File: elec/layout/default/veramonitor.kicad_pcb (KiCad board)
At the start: 2 copper layers, 111.2 x 70.4 mm, 109 parts, among them J1 ?, U1 ?, U10 ?, U11 ?, U12 ?, U13 ?, U14 ?, U15 ?, U16 ?, U17 ?, U18 ?, U19 ?, U2 ?, U20 ?, U21 ?, U22 ?, U23 ?, U24 ?, U25 ?, U26 ?, U27 ?, U28 ?, U29 ?, U3 ?, U30 ?, U31 ?, U32 ?, U33 ?, U34 ?, U35 ?, U36 ?, U37 ?, U38 ?, U39 ?, U4 ?, U40 ?, U41 ?, U42 ?, U43 ?, U44 ?, U45 ?, U46 ?, U47 ?, U48 ?, U49 ?, U5 ?, U50 ?, U51 ?, U6 ?, U7 ?, U8 ?, U9 ?

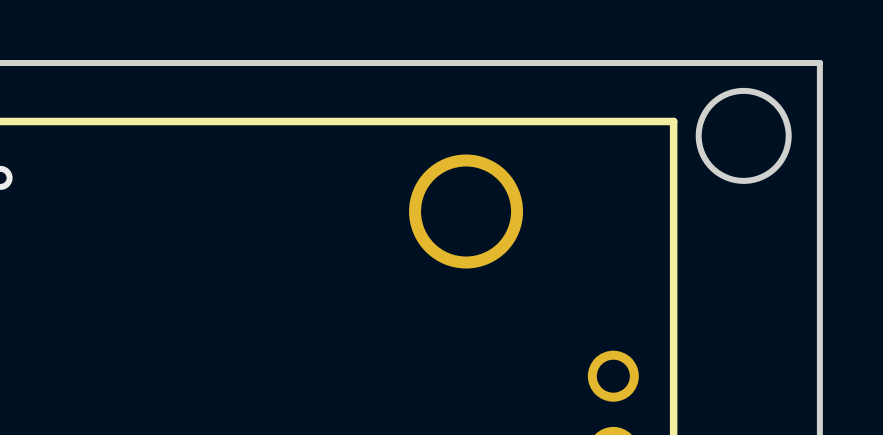
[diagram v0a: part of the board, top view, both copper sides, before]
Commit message: probs done
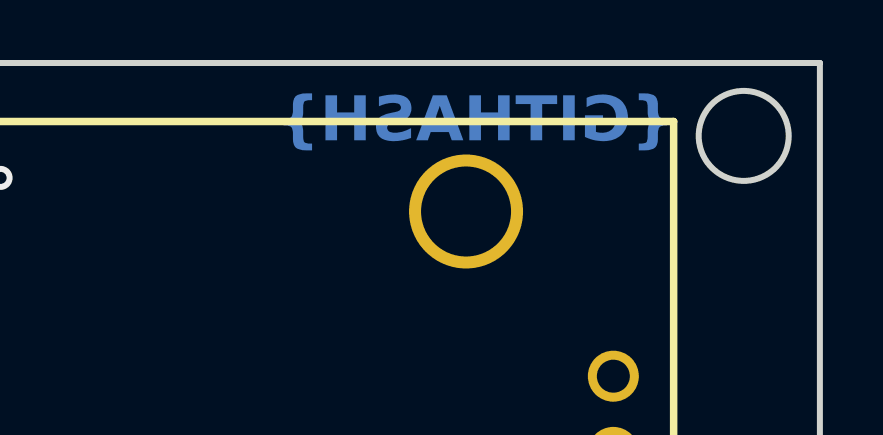
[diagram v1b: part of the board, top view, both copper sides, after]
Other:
- board text added: "{GITHASH}"
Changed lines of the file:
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@@
 		(layer "Edge.Cuts")
+	)
+	(gr_text "{GITHASH}"
+		(at 146.47 69.66 -0)
+		(layer "B.Cu")
+		(effects
+			(font
+				(size 1.5 1.5)
+				(thickness 0.3)
+				(bold yes)
+			)
+			(justify left bottom mirror)
+		)
 	)
 	(gr_text "AVERAGE\n"

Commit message: 11/8
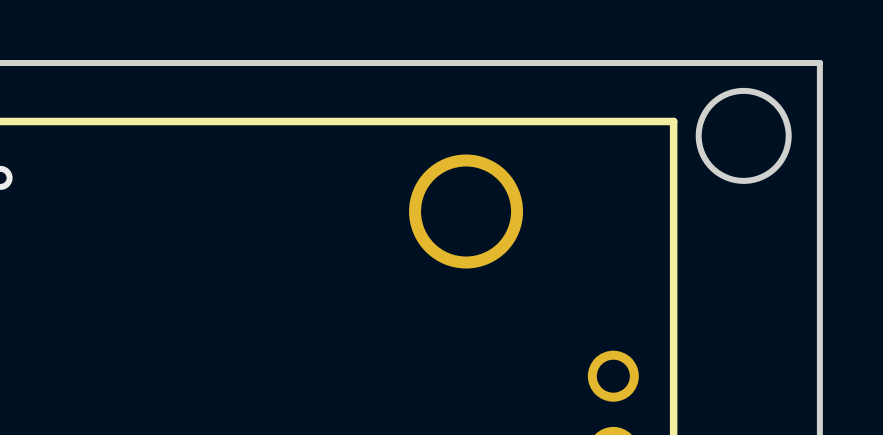
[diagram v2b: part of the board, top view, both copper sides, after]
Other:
- board text removed: "{GITHASH}"
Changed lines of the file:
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@@
 		(layer "Edge.Cuts")
-	)
-	(gr_text "{GITHASH}"
-		(at 146.47 69.66 -0)
-		(layer "B.Cu")
-		(effects
-			(font
-				(size 1.5 1.5)
-				(thickness 0.3)
-				(bold yes)
-			)
-			(justify left bottom mirror)
-		)
 	)
 	(gr_text "AVERAGE\n"
